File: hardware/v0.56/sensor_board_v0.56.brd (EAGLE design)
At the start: 50.8 x 50.8 mm, 67 parts, among them J3 USB-MICROB, U1 NEOPIXEL_NANO_2427, U10 TSL2591, U11 915MHz, U12 MH-Z19, U13 CCS811-I2C, U14 IAQ-CORE-C, U15 VLP-450-F, U16 VLP-450-F, U2 FT231XQ-R, U3 OPA344, U4 SI7021, U5 ATMEGA328P-MU, U6 ADMP401, U7 PMS7003, U8 MCP1703CB, U9 BMP280, X1 16 MHz

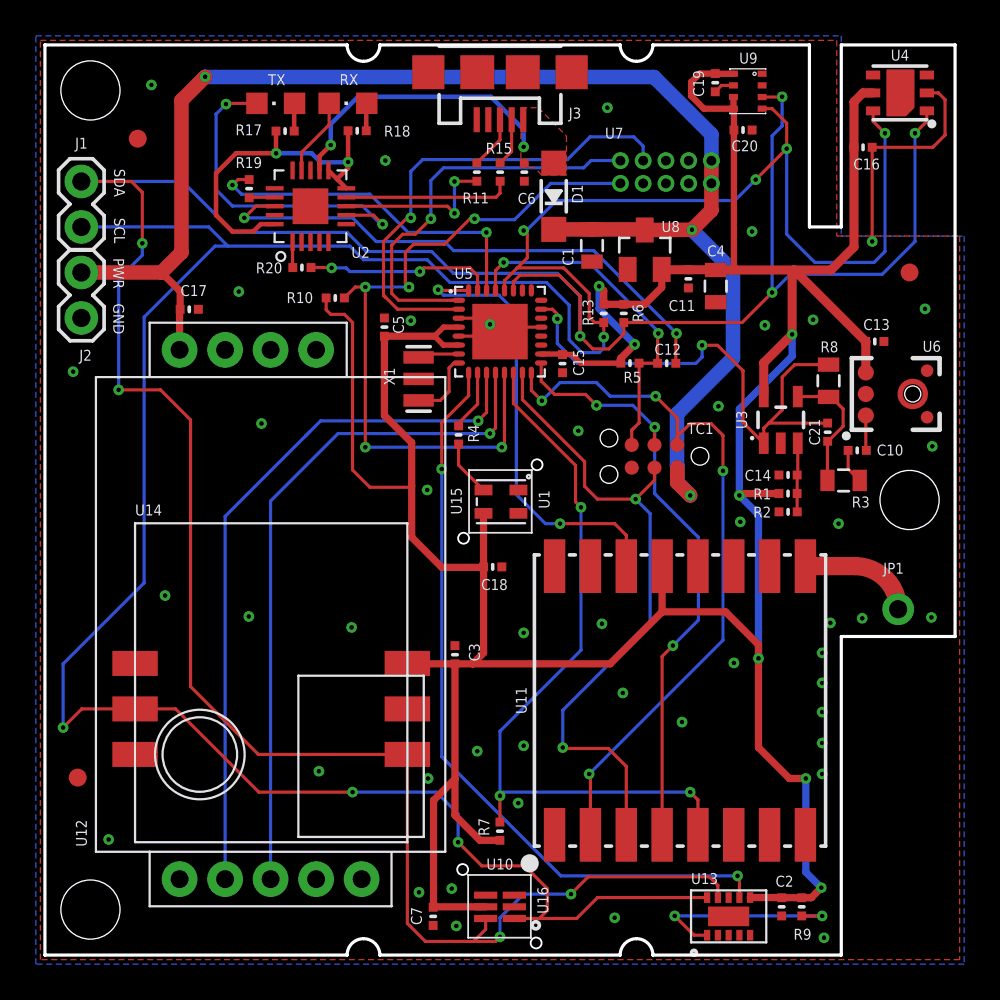
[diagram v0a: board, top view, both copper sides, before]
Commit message: v0.56b - minor update
- Moved CO2 sensor up the board
- Updated library for light pipe
- Adjusted components around the light pipe
- Some silkscreen and trace adjustments
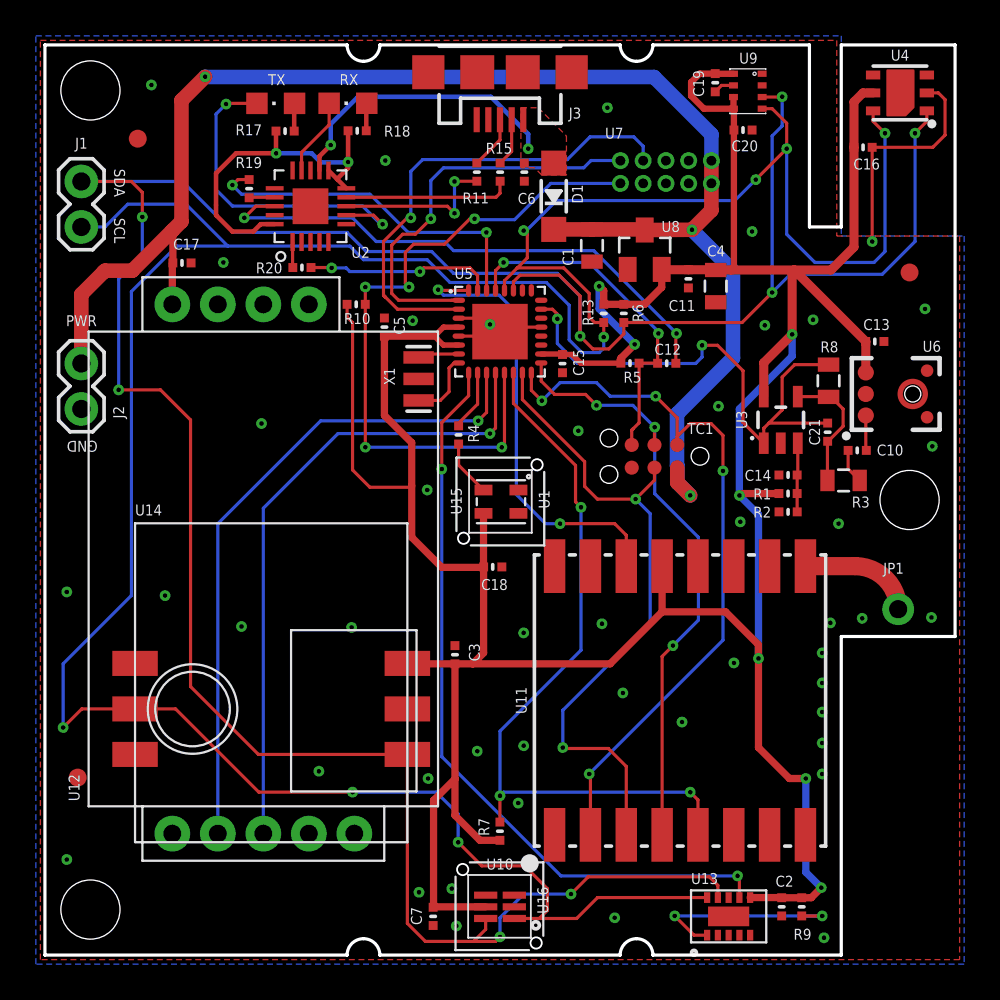
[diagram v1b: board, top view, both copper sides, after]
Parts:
- moved J2 5.08 mm to (2.03, 30.5)
- moved C17 2.62 mm to (7.65, 38.6)
- moved U12 2.57 mm to (2.44, 37.8)
- moved R10 1.22 mm to (17.4, 36.3)
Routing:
- net PWR: track 83.5 -> 86.3 mm
- net D7: track 39.8 -> 37.1 mm
- net D8: track 38.5 -> 36.1 mm
- net SCL: track 161.4 -> 163.7 mm
- net D9: track 40.3 -> 38.9 mm
- net VCC: track 200.9 -> 199.6 mm
